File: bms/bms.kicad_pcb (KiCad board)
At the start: 2 copper layers, 134 x 125 mm, 27 parts, among them J10 Conn_02x08_Odd_Even, J11 Conn_02x10_Odd_Even, J13 Conn_02x08_Odd_Even, J14 Conn_02x08_Odd_Even, J2 Conn_01x08_Socket, J22 Conn_02x10_Odd_Even, J3 Conn_01x06_Socket, J5 Conn_01x10_Socket, J6 Conn_01x06_Socket

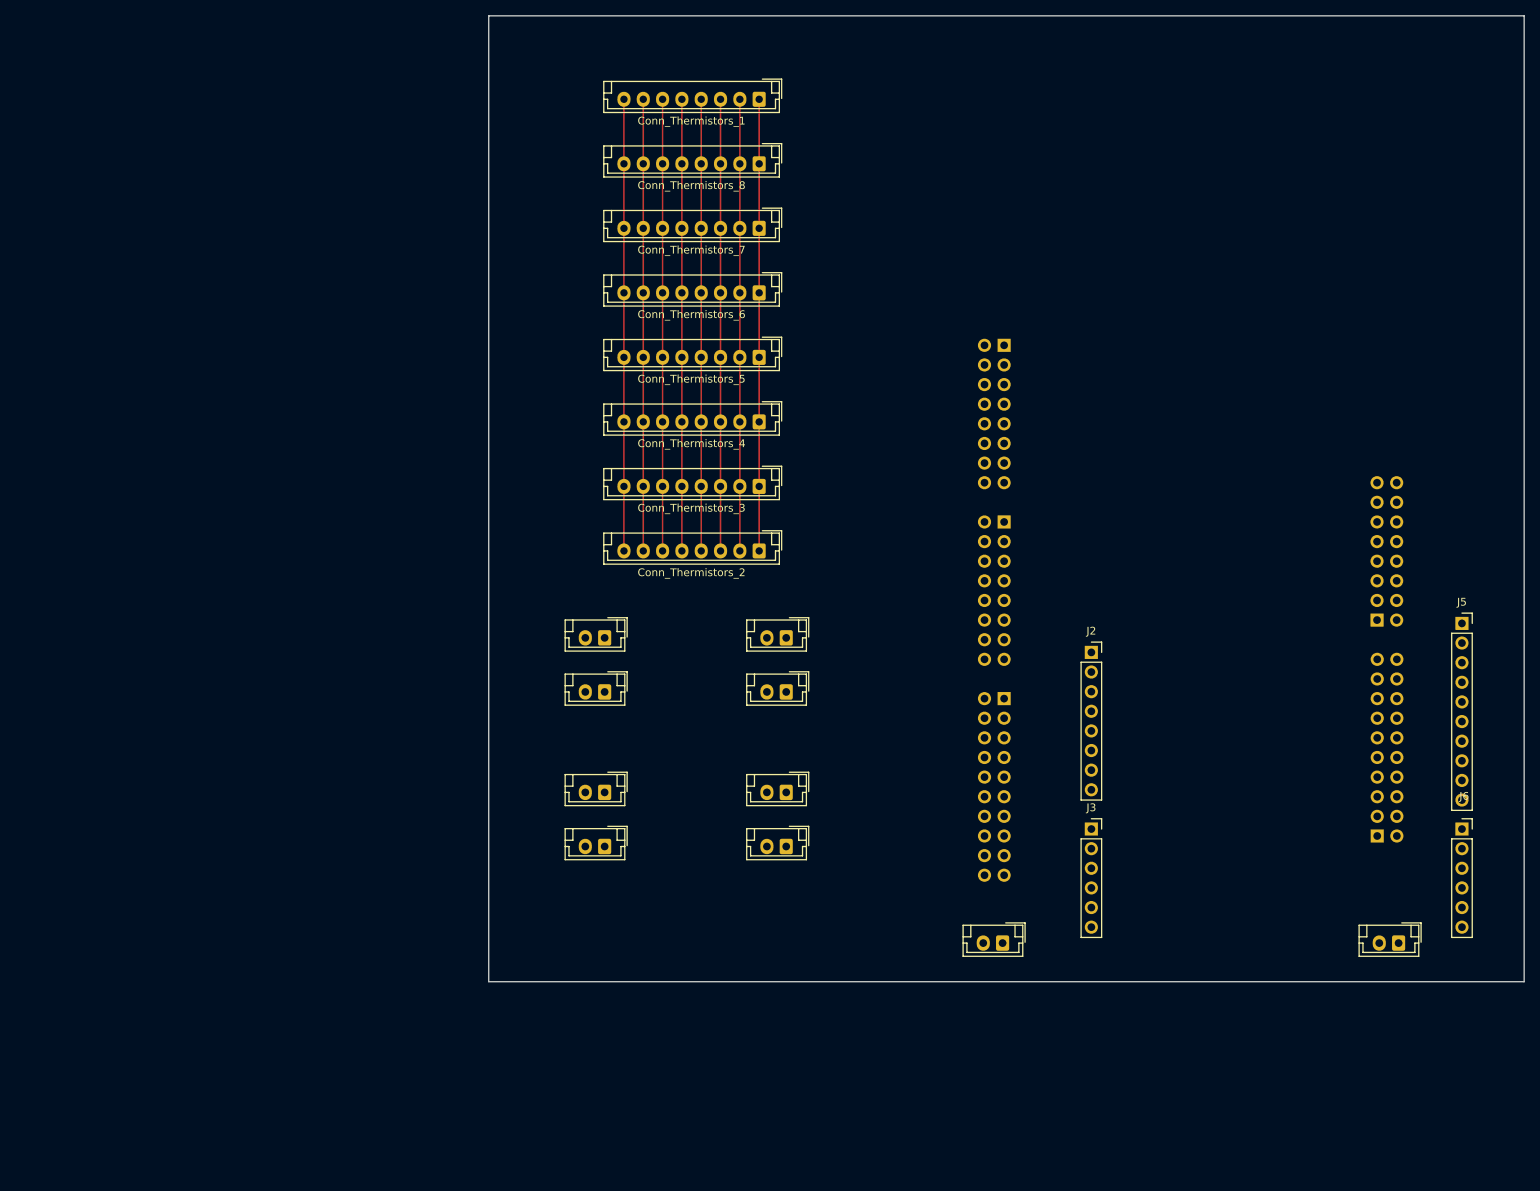
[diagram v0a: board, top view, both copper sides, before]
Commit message: v0.99
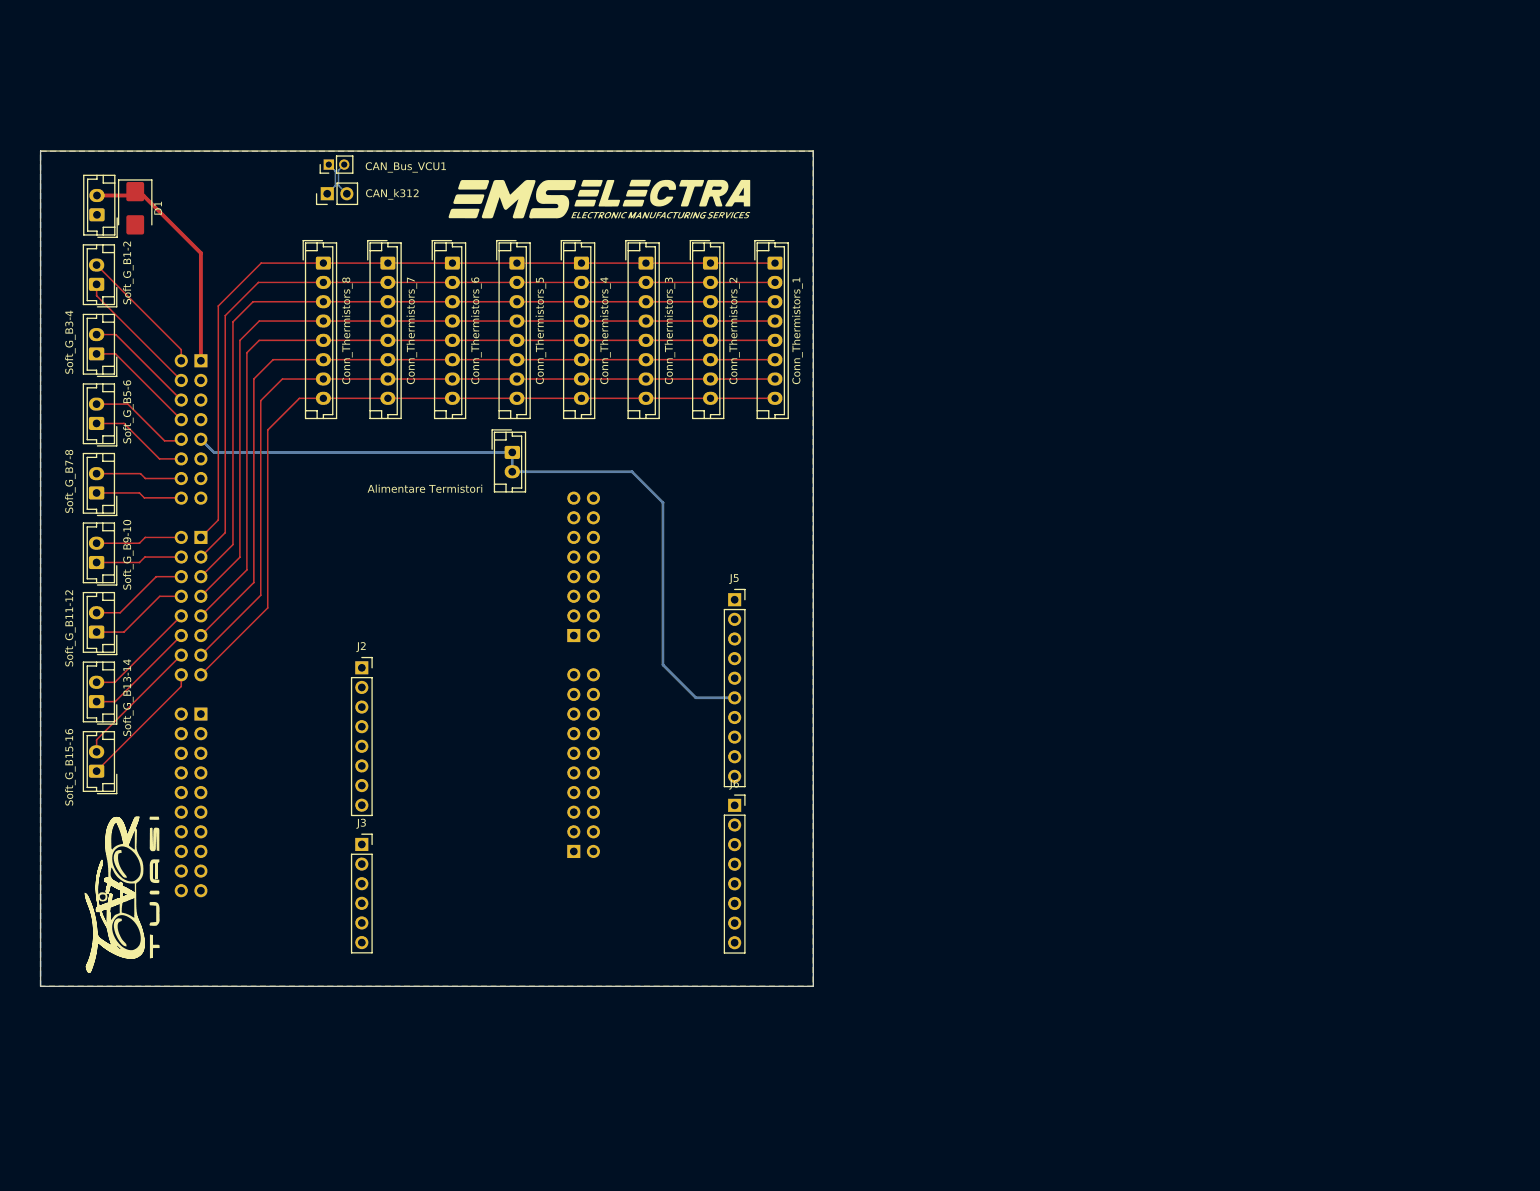
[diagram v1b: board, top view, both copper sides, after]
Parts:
- added CAN_Bus_VCU1: Conn_01x02_Pin, Connector_PinHeader_2.00mm:PinHeader_1x02_P2.00mm_Vertical, F.Cu at (93.3, 39.8)
- added CAN_k312: Conn_01x02_Pin, Connector_PinHeader_2.54mm:PinHeader_1x02_P2.54mm_Vertical, F.Cu at (93.1, 43.5)
- added D1: SS32, Diode_SMD:D_SMB, F.Cu at (68.2, 45.4)
- J6: value Conn_01x06_Socket -> Conn_01x08_Socket; footprint Connector_PinSocket_2.54mm:PinSocket_1x06_P2.54mm_Vertical -> Connector_PinSocket_2.54mm:PinSocket_1x08_P2.54mm_Vertical
- moved Battery1 150.4 mm to (63.3, 46.2), turned to 90 degrees
- moved Vdd1 131.1 mm to (117.0, 77.0), turned to -90 degrees
- moved J11 104.0 mm to (125.0, 128.6)
- moved J10 104.0 mm to (125.0, 100.7)
- moved J13 104.0 mm to (76.8, 65.1)
- moved J14 104.0 mm to (76.8, 88.0)
- moved J22 104.0 mm to (76.8, 110.9)
- moved J2 94.4 mm to (97.6, 104.9)
- moved J3 94.4 mm to (97.6, 127.7)
- moved J5 94.2 mm to (145.8, 96.1)
- moved J6 94.2 mm to (145.8, 122.7)
- moved Soft_G_B5-6 93.5 mm to (63.2, 73.2), turned to 90 degrees
- moved Soft_G_B7-8 92.9 mm to (63.2, 82.2), turned to 90 degrees
- moved Soft_G_B13-14 90.0 mm to (63.2, 109.2), turned to 90 degrees
- moved Soft_G_B15-16 89.8 mm to (63.2, 118.2), turned to 90 degrees
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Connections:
- J13 pad 1: unconnected-(J13-Pin_1-Pad1) -> Bat+
- J13 pad 10: unconnected-(J13-Pin_10-Pad10) -> G5
- J13 pad 12: unconnected-(J13-Pin_12-Pad12) -> G6
- J13 pad 13: unconnected-(J13-Pin_13-Pad13) -> GND
- J13 pad 14: unconnected-(J13-Pin_14-Pad14) -> G7
- J13 pad 16: unconnected-(J13-Pin_16-Pad16) -> G8
- J13 pad 2: unconnected-(J13-Pin_2-Pad2) -> G1
- J13 pad 4: unconnected-(J13-Pin_4-Pad4) -> G2
- J13 pad 6: unconnected-(J13-Pin_6-Pad6) -> G3
- J13 pad 8: unconnected-(J13-Pin_8-Pad8) -> G4
- J13 pad 9: unconnected-(J13-Pin_9-Pad9) -> Vdd
- J14 pad 1: unconnected-(J14-Pin_1-Pad1) -> 1
- J14 pad 10: unconnected-(J14-Pin_10-Pad10) -> G13
- J14 pad 11: unconnected-(J14-Pin_11-Pad11) -> 6
- J14 pad 12: unconnected-(J14-Pin_12-Pad12) -> G14
- J14 pad 13: unconnected-(J14-Pin_13-Pad13) -> 7
- J14 pad 14: unconnected-(J14-Pin_14-Pad14) -> G15
- J14 pad 15: unconnected-(J14-Pin_15-Pad15) -> 8
- J14 pad 16: unconnected-(J14-Pin_16-Pad16) -> G16
- J14 pad 2: unconnected-(J14-Pin_2-Pad2) -> G9
- J14 pad 3: unconnected-(J14-Pin_3-Pad3) -> 2
- J14 pad 4: unconnected-(J14-Pin_4-Pad4) -> G10
- J14 pad 5: unconnected-(J14-Pin_5-Pad5) -> 3
- J14 pad 6: unconnected-(J14-Pin_6-Pad6) -> G11
- J14 pad 7: unconnected-(J14-Pin_7-Pad7) -> 4
- J14 pad 8: unconnected-(J14-Pin_8-Pad8) -> G12
- J14 pad 9: unconnected-(J14-Pin_9-Pad9) -> 5
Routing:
- net Vdd: track 0.00 -> 96.7 mm
- net 3: track 58.5 -> 105.9 mm
- net 5: track 58.5 -> 105.5 mm
- net 4: track 58.5 -> 105.5 mm
- net 2: track 58.5 -> 105.5 mm
- net 1: track 58.5 -> 105.2 mm
- net 6: track 58.5 -> 104.5 mm
- net 7: track 58.5 -> 103.9 mm
- net 8: track 58.5 -> 102.6 mm
- net Bat+: track 0.00 -> 30.5 mm
- net G15: track 0.00 -> 17.0 mm
- net G16: track 0.00 -> 17.0 mm
- net G2: track 0.00 -> 17.0 mm
- net G1: track 0.00 -> 16.9 mm
- net G13: track 0.00 -> 14.5 mm
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- added copper zone on B.Cu, net GND
- added copper zone on F.Cu, net GND
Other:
- board size 134 x 125 mm -> 100 x 108.1 mm

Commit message: V0.999 a little more polished
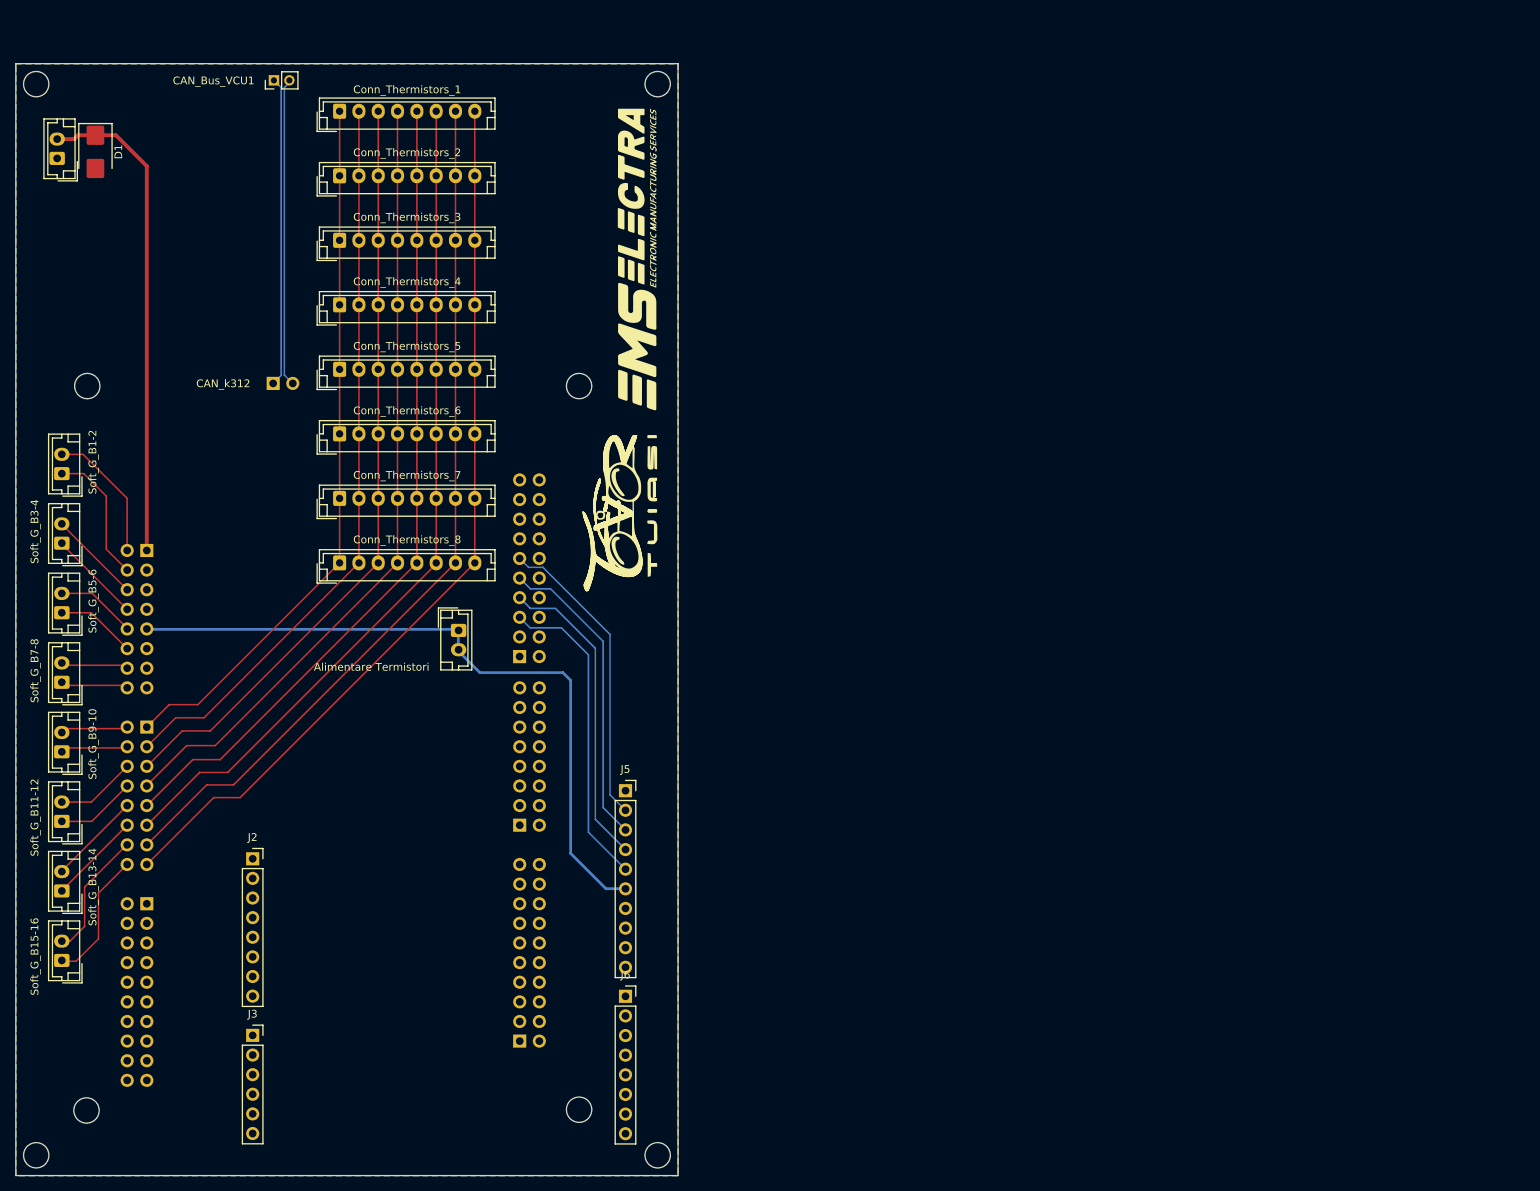
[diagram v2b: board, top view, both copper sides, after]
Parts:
- added J10: Conn_02x10_Odd_Even, Connector_PinHeader_2.54mm:PinHeader_2x10_P2.54mm_Vertical, B.Cu at (118.0, 103.4)
- CAN_k312: moved to B.Cu
- moved Conn_Thermistors_2 59.7 mm to (94.7, 32.9), turned to 0 degrees
- moved Conn_Thermistors_3 49.3 mm to (94.7, 41.2), turned to 0 degrees
- moved Conn_Thermistors_4 39.8 mm to (94.7, 49.5), turned to 0 degrees
- moved Conn_Thermistors_1 38.9 mm to (94.7, 91.3), turned to 0 degrees
- moved Conn_Thermistors_5 31.8 mm to (94.7, 57.9), turned to 0 degrees
- moved Conn_Thermistors_8 31.1 mm to (94.7, 83.0), turned to 0 degrees
- moved J3 28.5 mm to (83.5, 152.4)
- moved J5 28.5 mm to (131.7, 120.8)
- moved J6 28.5 mm to (131.7, 147.4)
- moved J2 28.5 mm to (83.5, 129.6)
- moved Conn_Thermistors_6 26.8 mm to (94.7, 66.2), turned to 0 degrees
- moved Conn_Thermistors_7 26.5 mm to (94.7, 74.6), turned to 0 degrees
- moved J11 25.5 mm to (118.0, 125.2)
- moved J12 25.5 mm to (118.0, 153.2)
- moved J13 25.5 mm to (69.8, 89.7)
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- renumbered J10 to J11, J11 to J12, J22 to J15
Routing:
- net SCK: track 0.00 -> 40.6 mm
- net MISO: track 0.00 -> 40.2 mm
- net SOUT: track 0.00 -> 39.8 mm
- net CS: track 0.00 -> 39.4 mm
- net CAN_L_k: track 4.56 -> 40.1 mm
- net CAN_H_k: track 4.54 -> 39.9 mm
- net Bat+: track 30.5 -> 63.2 mm
- net 8: track 102.6 -> 117.1 mm
- net 1: track 105.2 -> 92.2 mm
- net 2: track 105.5 -> 95.8 mm
- net 7: track 103.9 -> 113.5 mm
- net 3: track 105.9 -> 99.3 mm
- net Vdd: track 96.7 -> 90.5 mm
- net 6: track 104.5 -> 110.1 mm
- net G5: track 13.0 -> 10.4 mm
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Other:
- board size 100 x 108.1 mm -> 85.7 x 143.9 mm
